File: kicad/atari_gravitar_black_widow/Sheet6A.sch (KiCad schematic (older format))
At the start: 10 parts

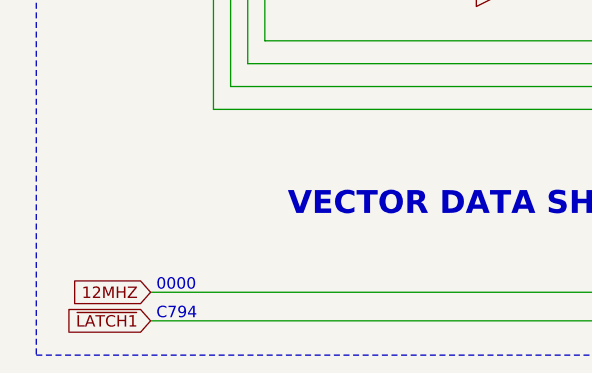
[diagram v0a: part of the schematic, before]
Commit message: Completed sheet 6B
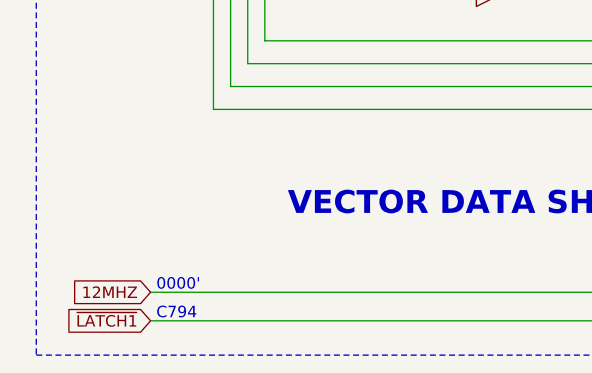
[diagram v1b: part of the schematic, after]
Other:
- note added: "0000'"
- note removed: "0000"
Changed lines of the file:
@@
 $EndComp
 Text Notes 5750 13900 0    50   ~ 0
-0000
+0000'
 Text Notes 5750 14025 0    50   ~ 0
 C794
